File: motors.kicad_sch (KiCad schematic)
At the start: 12 parts, among them U8 DRV8874PWPR, U9 DRV8874PWPR

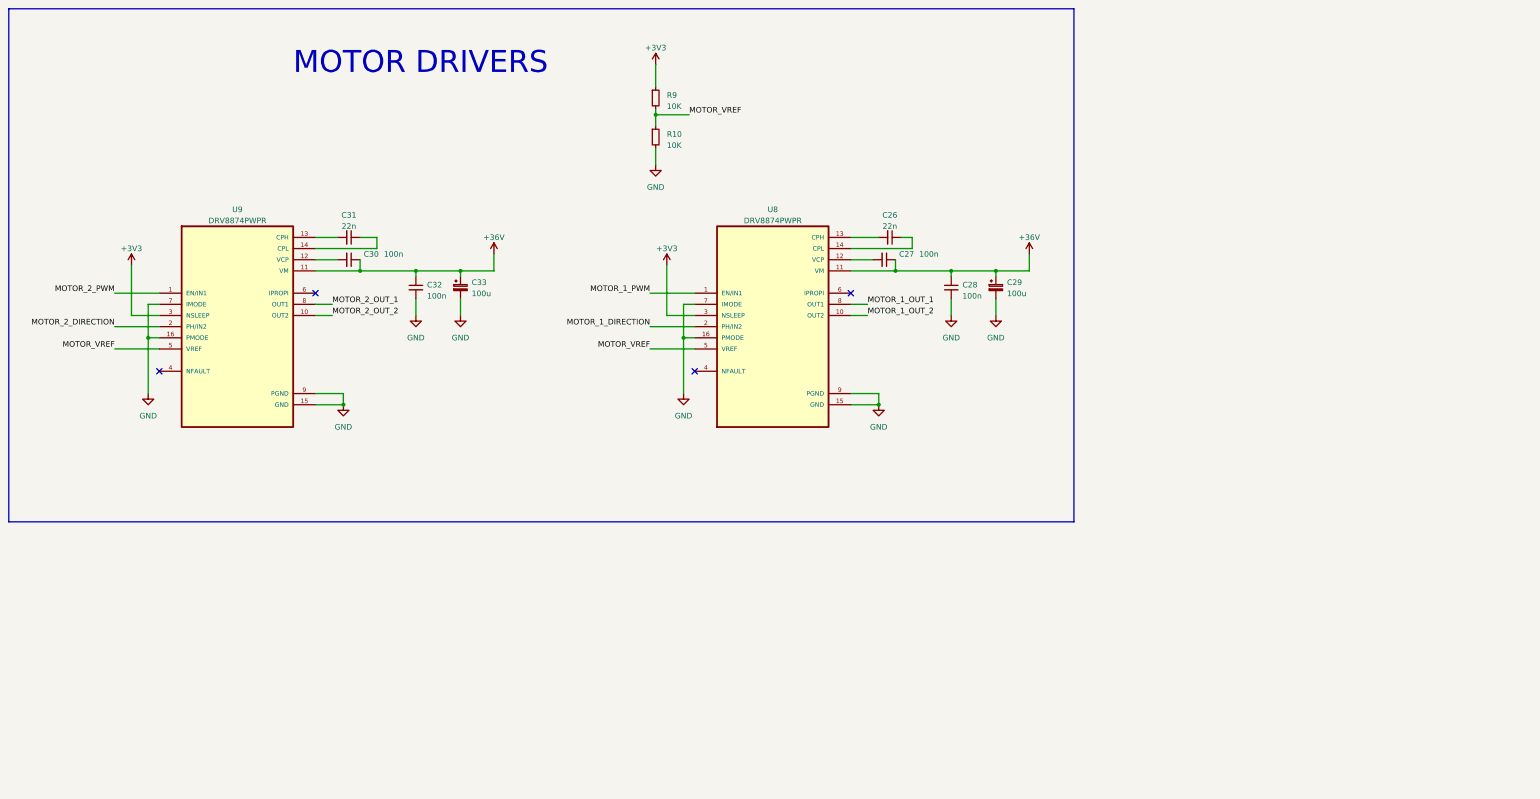
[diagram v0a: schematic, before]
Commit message: Update placement
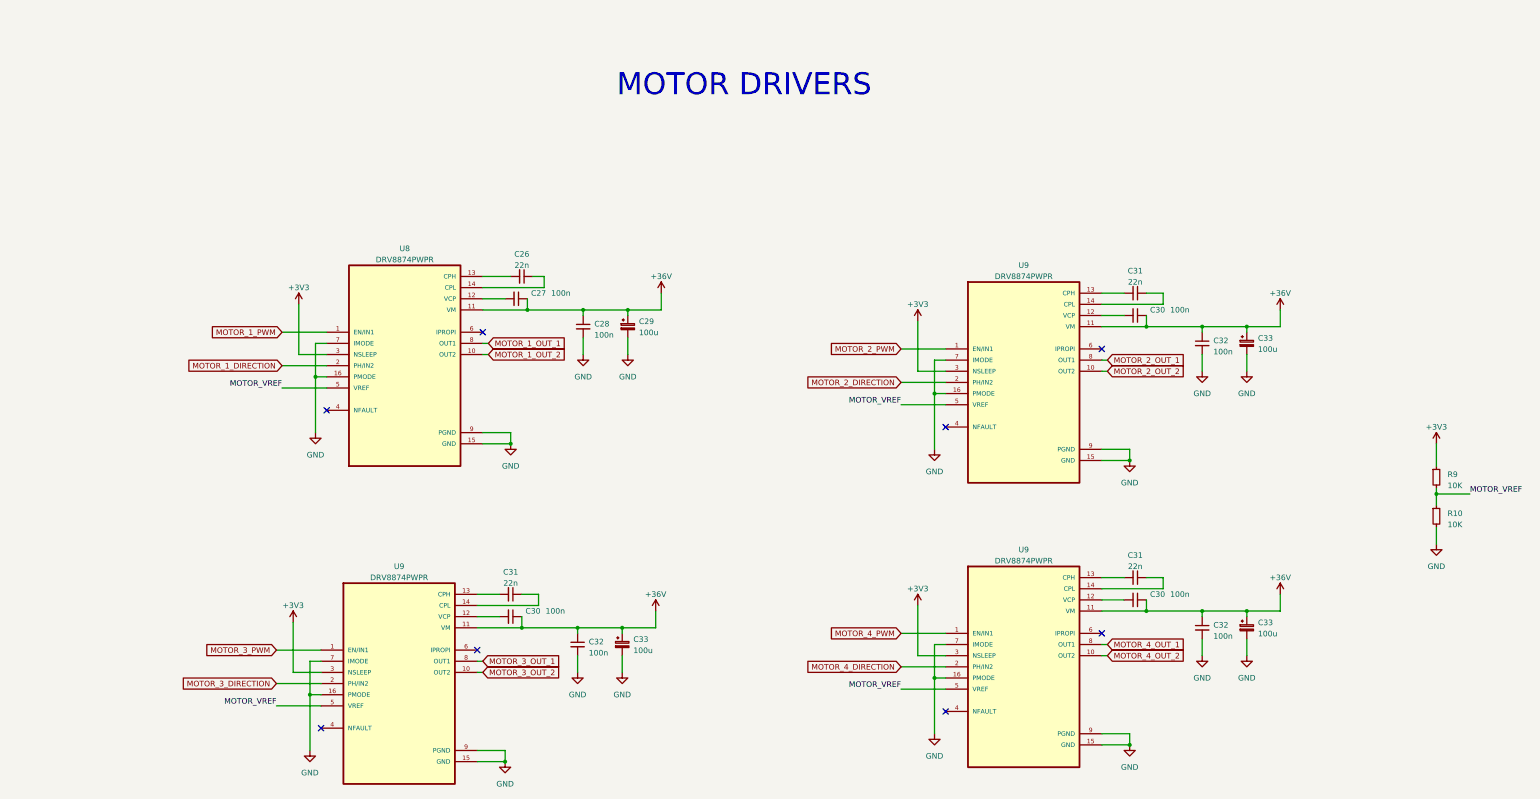
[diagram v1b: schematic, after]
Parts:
- added C30 (x2), C32 (x2): 100n, Capacitor_SMD:C_0402_1005Metric, symbol Device:C_Small
- added C31 (x2): 22n, Capacitor_SMD:C_0402_1005Metric, symbol Device:C_Small
- added C33 (x2): 100u, Capacitor_SMD:C_0805_2012Metric, symbol Device:C_Polarized_Small
- added U9 (x2): DRV8874PWPR, Libraries:SOP65P640X120-17N, symbol DRV8874PWPR:DRV8874PWPR
- C26, C27, C28, C30, C31, C32: footprint Capacitor_SMD:C_0603_1608Metric -> Capacitor_SMD:C_0402_1005Metric
- C29, C33: footprint Capacitor_SMD:C_0603_1608Metric -> Capacitor_SMD:C_0805_2012Metric
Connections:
- net +36V: now also C30.1, C30.1, C32.1, C32.1, C33.1, C33.1, U9.11 (VM), U9.11 (VM)
- net +3V3: now also U9.3 (NSLEEP), U9.3 (NSLEEP)
- net GND: now also C32.2, C32.2, C33.2, C33.2, U9.15 (GND), U9.15 (GND), U9.16 (PMODE), U9.16 (PMODE), U9.7 (IMODE), U9.7 (IMODE), U9.9 (PGND), U9.9 (PGND)
- net MOTOR_VREF: now also U9.5 (VREF), U9.5 (VREF)
- new net: C30.2, U9.12 (VCP) (x2)
- new net: C31.2, U9.13 (CPH) (x2)
- new net: C31.1, U9.14 (CPL) (x2)
- new net MOTOR_3_DIRECTION: U9.2 (PH/IN2)
- new net MOTOR_3_OUT_1: U9.8 (OUT1)
- new net MOTOR_3_OUT_2: U9.10 (OUT2)
- new net MOTOR_3_PWM: U9.1 (EN/IN1)
- new net MOTOR_4_DIRECTION: U9.2 (PH/IN2)
- new net MOTOR_4_OUT_1: U9.8 (OUT1)
- new net MOTOR_4_OUT_2: U9.10 (OUT2)
- new net MOTOR_4_PWM: U9.1 (EN/IN1)
- no-connect marks 4 -> 8
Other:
- moved on the sheet: C26, C27, C28, C29, C30, C31, C32, C33, R10, R9, U8, U9
